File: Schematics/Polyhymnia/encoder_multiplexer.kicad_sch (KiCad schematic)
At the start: 4 parts, among them J7 Serial-Out, U6 ATmega32-16P, U8 74HC595, U9 74HC595

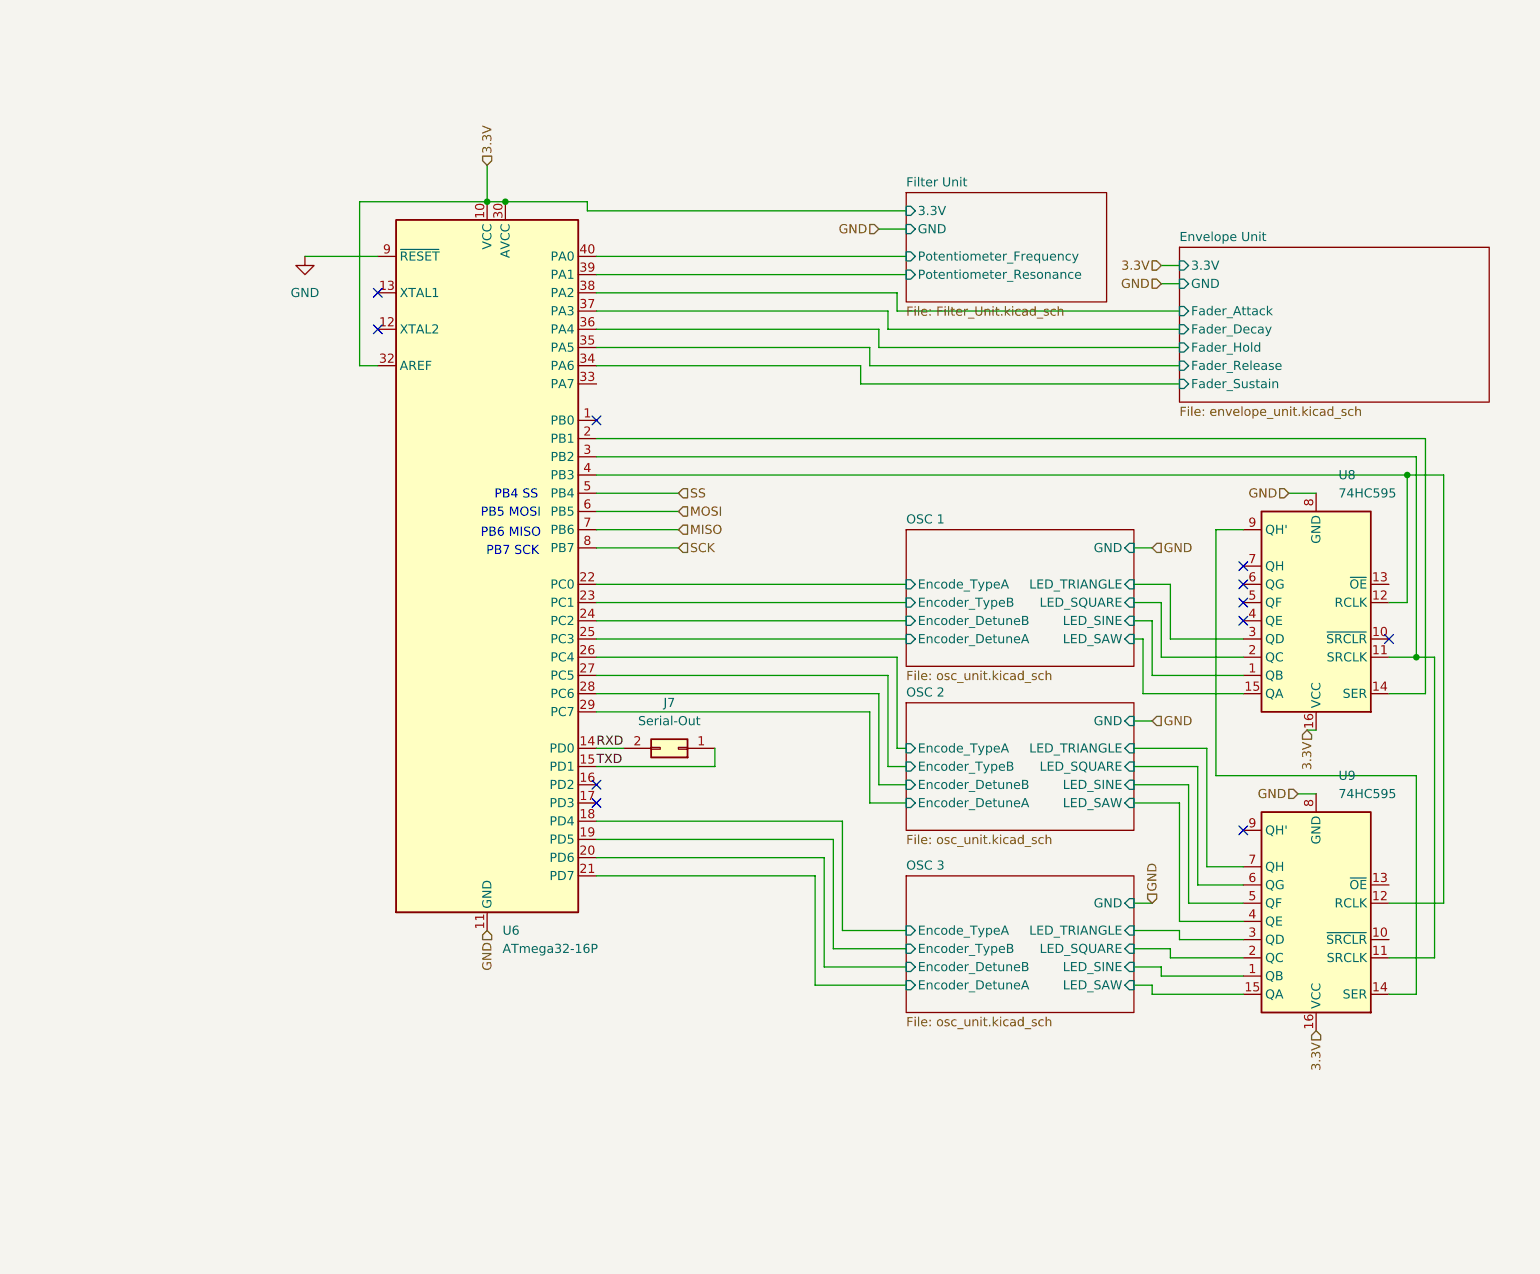
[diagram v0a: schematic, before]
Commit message: Merge
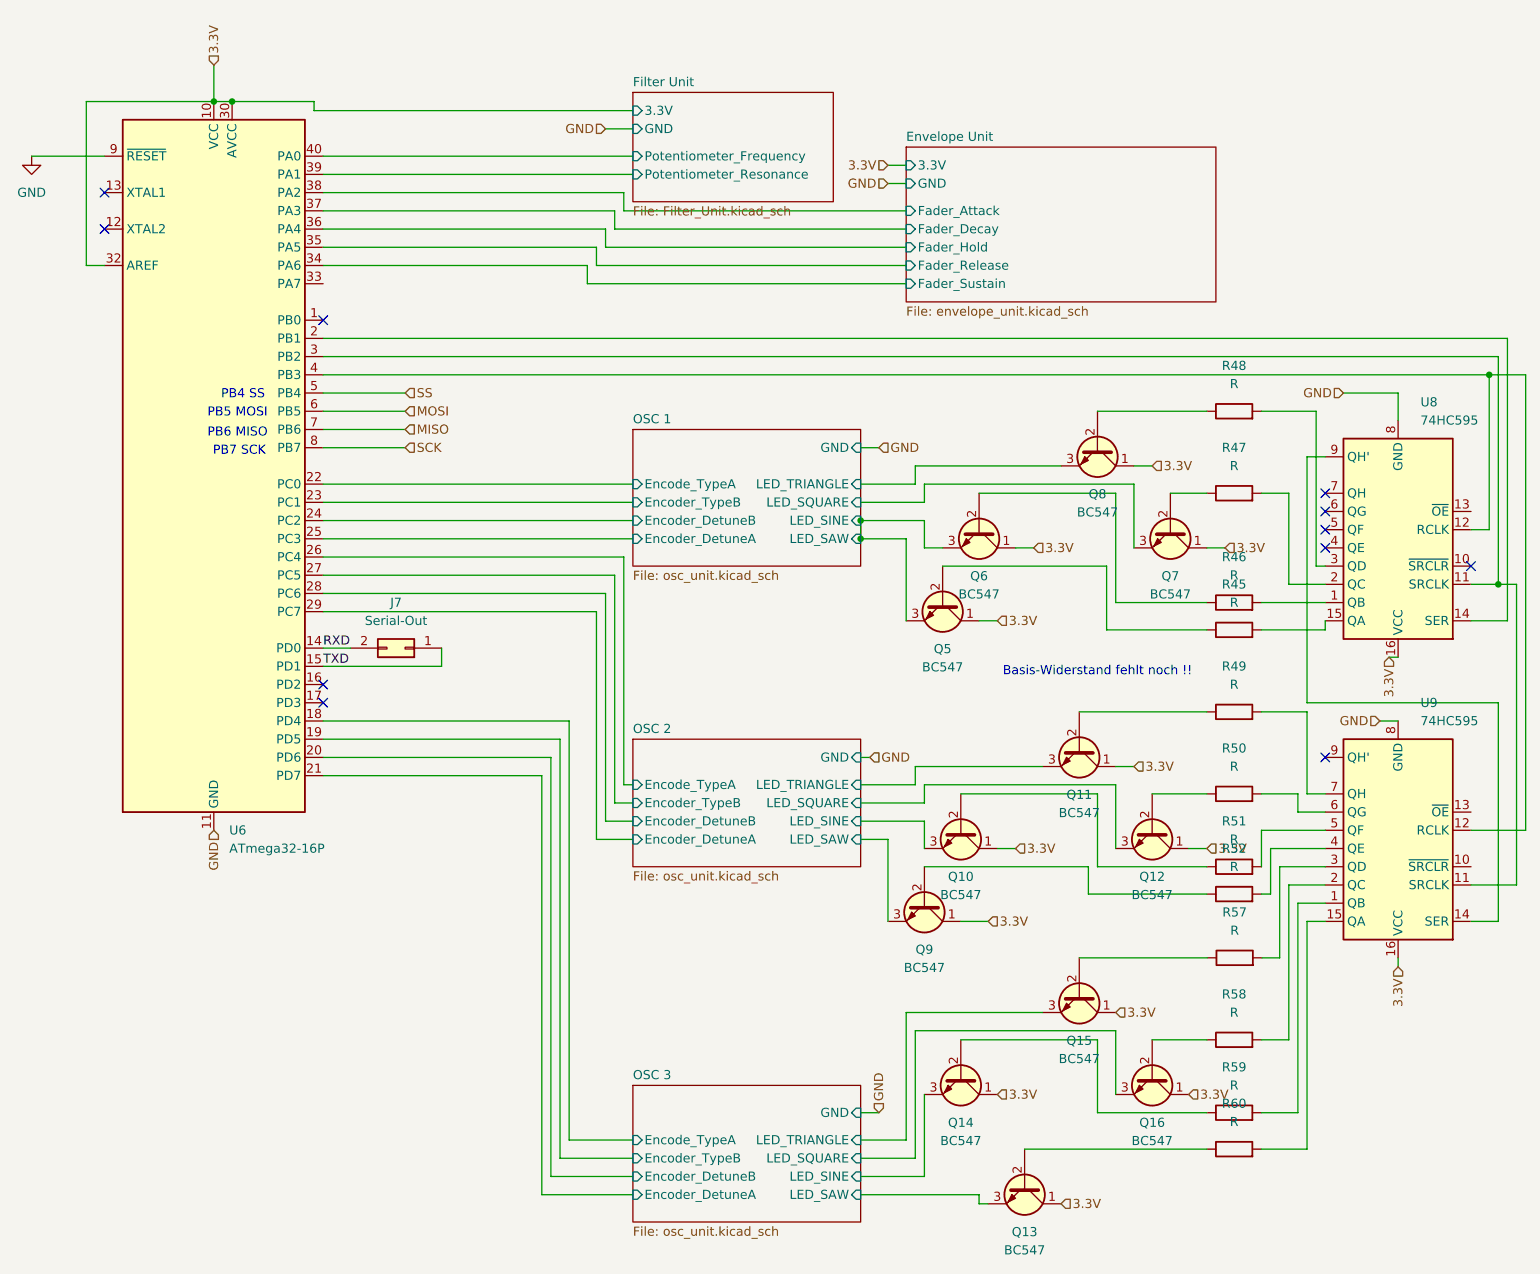
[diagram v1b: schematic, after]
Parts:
- added Q10, Q11, Q12, Q13, Q14, Q15, Q16, Q5, Q6, Q7, Q8, Q9: BC547, PCM_Package_TO_SOT_THT_AKL:TO-92_Inline_Wide_CBE, symbol PCM_Transistor_BJT_AKL:BC547
- added R45, R46, R47, R48, R49, R50, R51, R52, R57, R58, R59, R60: R, symbol Device:R
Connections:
- net 3.3V: now also Q10.1 (C), Q11.1 (C), Q12.1 (C), Q13.1 (C), Q14.1 (C), Q15.1 (C), Q16.1 (C), Q5.1 (C), Q6.1 (C), Q7.1 (C), Q8.1 (C), Q9.1 (C)
- net OSC 1/LED_SAW: now also Q5.3 (E), Q6.3 (E); no longer U8.15 (QA)
- net OSC 1/LED_SQUARE: now also Q7.3 (E); no longer U8.2 (QC)
- net OSC 1/LED_TRIANGLE: now also Q8.3 (E); no longer U8.3 (QD)
- net OSC 2/LED_SAW: now also Q9.3 (E); no longer U9.4 (QE)
- net OSC 2/LED_SINE: now also Q10.3 (E); no longer U9.5 (QF)
- net OSC 2/LED_SQUARE: now also Q12.3 (E); no longer U9.6 (QG)
- net OSC 2/LED_TRIANGLE: now also Q11.3 (E); no longer U9.7 (QH)
- net OSC 3/LED_SAW: now also Q13.3 (E); no longer U9.15 (QA)
- net OSC 3/LED_SINE: now also Q14.3 (E); no longer U9.1 (QB)
- net OSC 3/LED_SQUARE: now also Q16.3 (E); no longer U9.2 (QC)
- net OSC 3/LED_TRIANGLE: now also Q15.3 (E); no longer U9.3 (QD)
- net OSC 1/LED_SINE: no longer names the net of U8.1 (QB)
- net OSC 1/LED_SINE: now also R46.2
- new net: Q10.2 (B), R51.1
- new net: Q12.2 (B), R50.1
- new net: R50.2, U9.6 (QG)
- new net: Q9.2 (B), R52.1
- new net: R52.2, U9.4 (QE)
- new net: Q14.2 (B), R59.1
- new net: Q6.2 (B), R46.1
- new net: R45.2, U8.15 (QA)
- new net: R47.2, U8.2 (QC)
- new net: R48.2, U8.3 (QD)
- new net: Q7.2 (B), R47.1
- new net: Q13.2 (B), R60.1
- new net: Q16.2 (B), R58.1
- new net: Q15.2 (B), R57.1
- new net: R57.2, U9.3 (QD)
- new net: R59.2, U9.1 (QB)
- new net: R60.2, U9.15 (QA)
- new net: R58.2, U9.2 (QC)
- new net: R51.2, U9.5 (QF)
- new net: R49.2, U9.7 (QH)
- new net: Q11.2 (B), R49.1
- new net: Q5.2 (B), R45.1
- new net: Q8.2 (B), R48.1
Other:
- note added: "Basis-Widerstand fehlt noch !!"
- title: (none) -> Encoder Control Unit
- moved on the sheet: J7, U6, U8, U9
